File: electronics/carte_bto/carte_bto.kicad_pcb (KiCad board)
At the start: 2 copper layers, 160 x 100 mm, 190 parts, among them J1 DIN41612_02x32_AB, J2 Conn_01x01, J3 Conn_01x01, J4 Conn_01x01, J5 Conn_01x01, J6 Conn_01x01, Q1 MMBT2222A, Q10 MMBT2222A, Q11 MMBT2222A, Q12 MMBT2222A, Q13 MMBT2222A, Q14 MMBT2222A, Q15 MMBT2222A, Q16 MMBT2222A, Q17 MMBT2222A, Q18 MMBT2222A, Q2 MMBT2222A, Q3 MMBT2222A, Q4 MMBT2222A, Q5 MMBT2222A, Q6 MMBT2222A, Q7 MMBT2222A, Q8 MMBT2222A, Q9 MMBT2222A, U1 74AHC541, U2 LTC1859IG_PBF, U3 LT6654AIS6-2.5_TRPBF, U4 74AHC541, U5 L78L05_SOT89

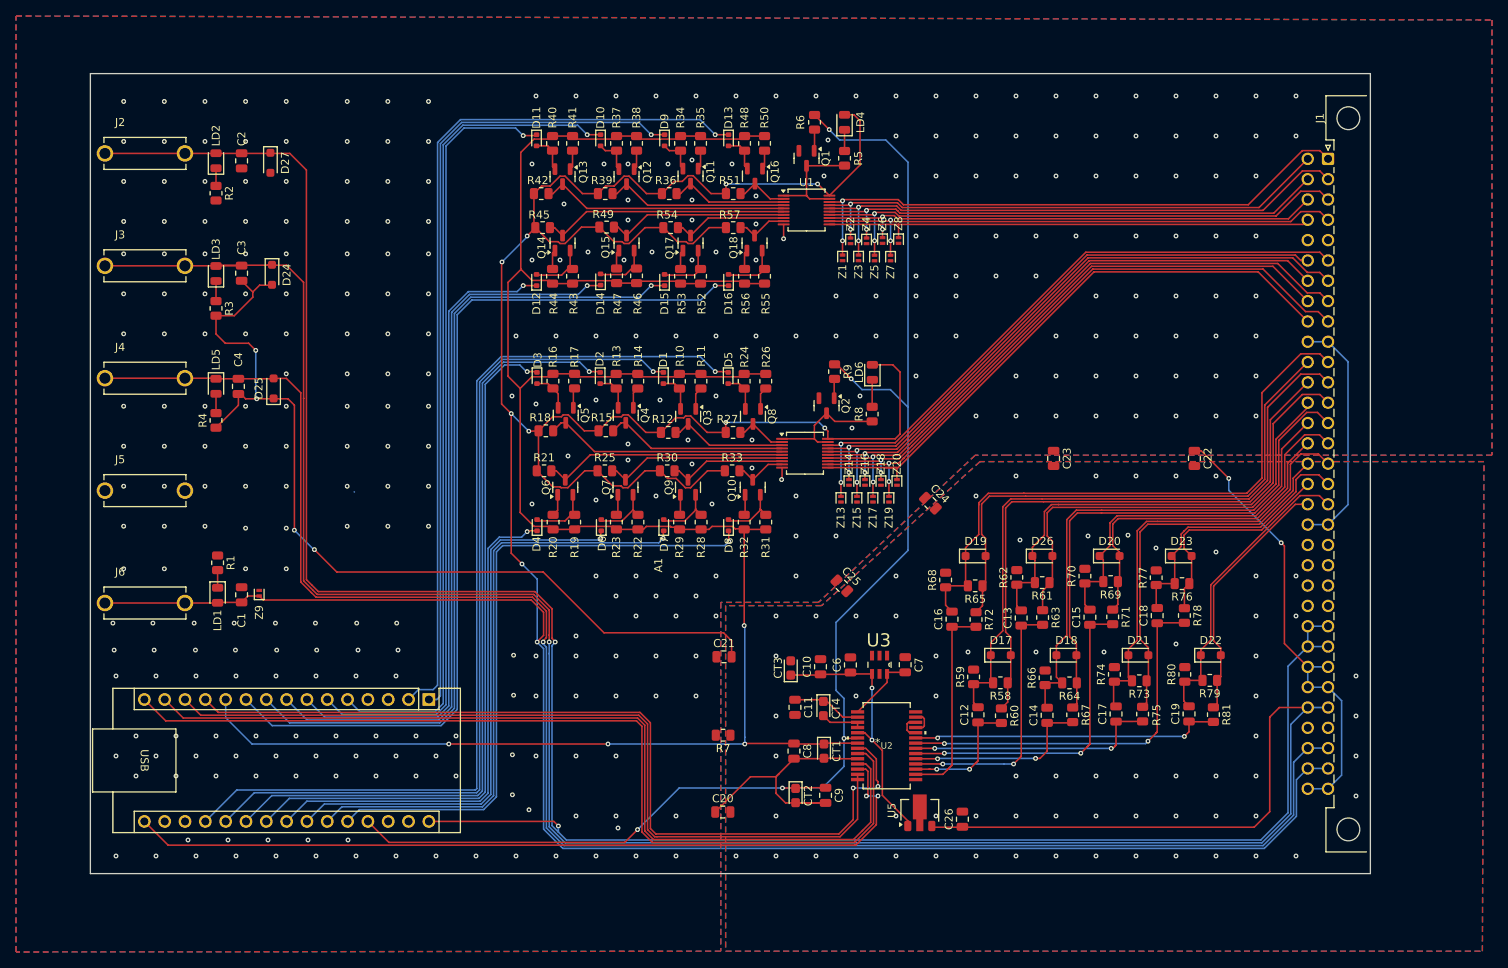
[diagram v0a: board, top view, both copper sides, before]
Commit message: BTO: Better routing.
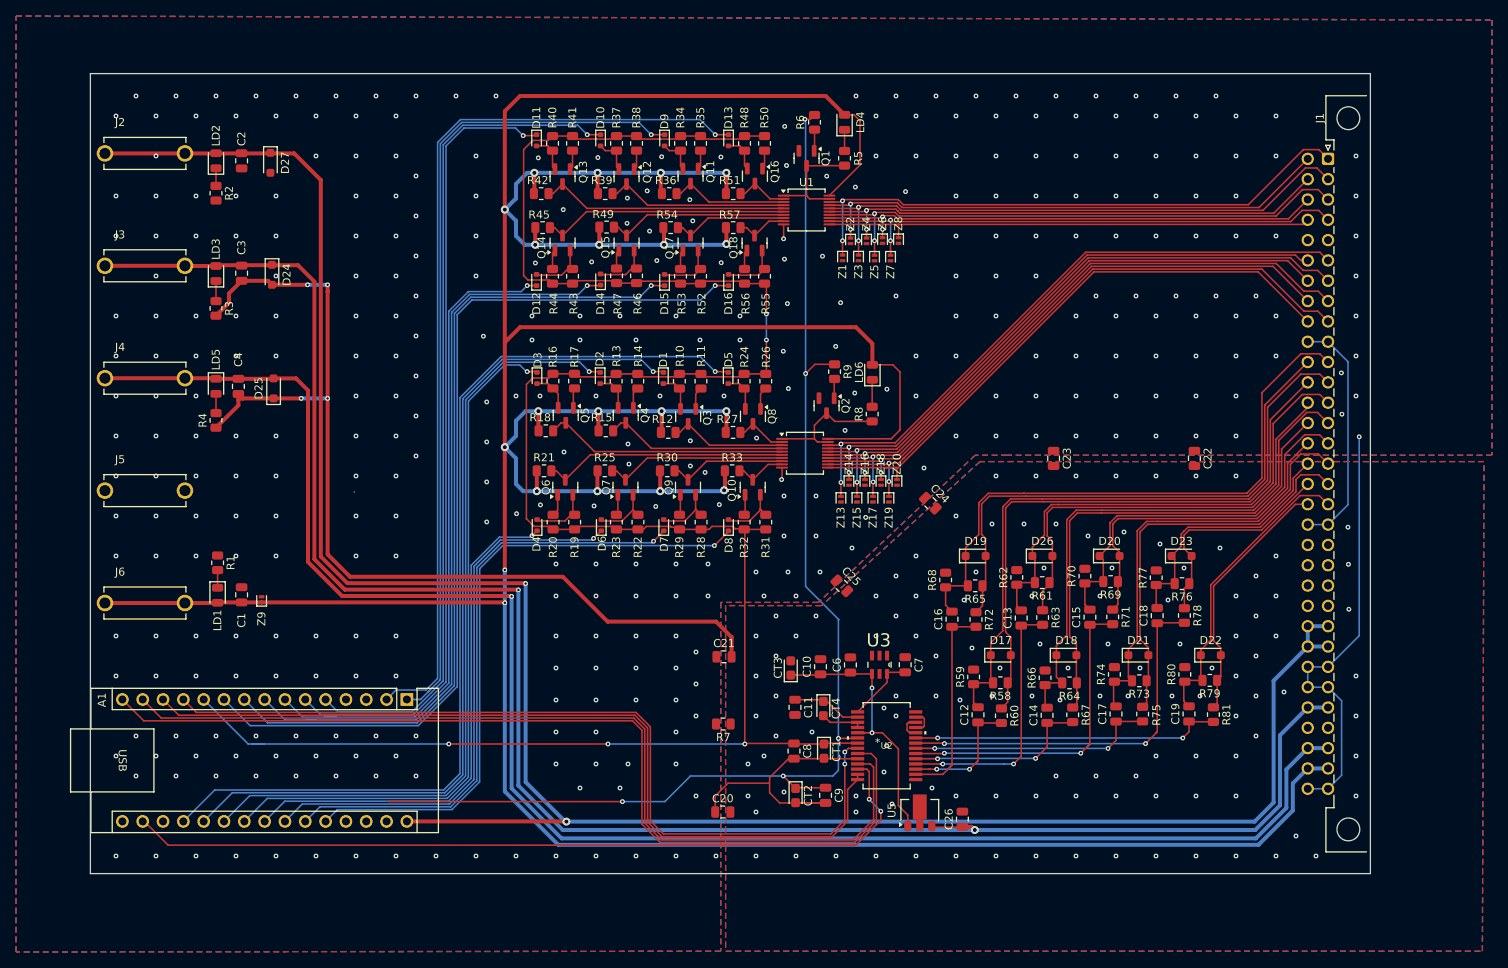
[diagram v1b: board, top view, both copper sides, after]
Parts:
- moved A1 2.75 mm to (96.4, 117.9)
- moved R7 1.40 mm to (135.9, 121.0)
- moved Z9 0.85 mm to (78.2, 105.5)
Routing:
- net +5V: track 437.8 -> 538.0 mm, vias 10 -> 20
- net +15V: track 297.0 -> 233.5 mm, vias 1 -> 2
- net +5VARD: track 176.1 -> 154.5 mm
- net GND1: track 151.0 -> 160.2 mm, vias 74 -> 126
- net -15V: track 215.1 -> 209.8 mm
- net +12VP: track 277.7 -> 272.6 mm
- net /SPI.cipo: track 117.4 -> 120.0 mm
- net /SPI.copi: track 112.7 -> 115.2 mm
- net /data4: track 80.9 -> 83.4 mm
- net /adc_busy: track 110.0 -> 107.5 mm
- net /data1: track 100.4 -> 102.8 mm
- net /data0: track 110.5 -> 112.8 mm
- net /data5: track 91.6 -> 93.8 mm
- net /ioref: track 271.1 -> 269.0 mm, vias 4 -> 5
- net GND2: track 93.8 -> 91.8 mm, vias 346 -> 367
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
